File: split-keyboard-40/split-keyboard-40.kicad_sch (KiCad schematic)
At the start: 85 parts, among them SW1 Switch, SW10 Switch, SW11 Switch, SW12 Switch, SW13 Switch, SW14 Switch, SW15 Switch, SW16 Switch, SW17 Switch, SW18 Switch, SW19 Switch, SW2 Switch, SW20 Switch, SW21 Switch, SW22 Switch, SW23 Switch, SW24 Switch, SW25 Switch, SW26 Switch, SW27 Switch, SW28 Switch, SW29 Switch, SW3 Switch, SW30 Switch, SW31 Switch, SW32 Switch, SW33 Switch, SW34 Switch, SW35 Switch, SW36 Switch, SW37 Switch, SW38 Switch, SW39 Switch, SW4 Switch, SW40 Switch, SW41 Switch, SW42 Switch, SW5 Switch, SW6 Switch, SW7 Switch, SW8 Switch, SW9 Switch, U1 Raspberry_Pi_Pico

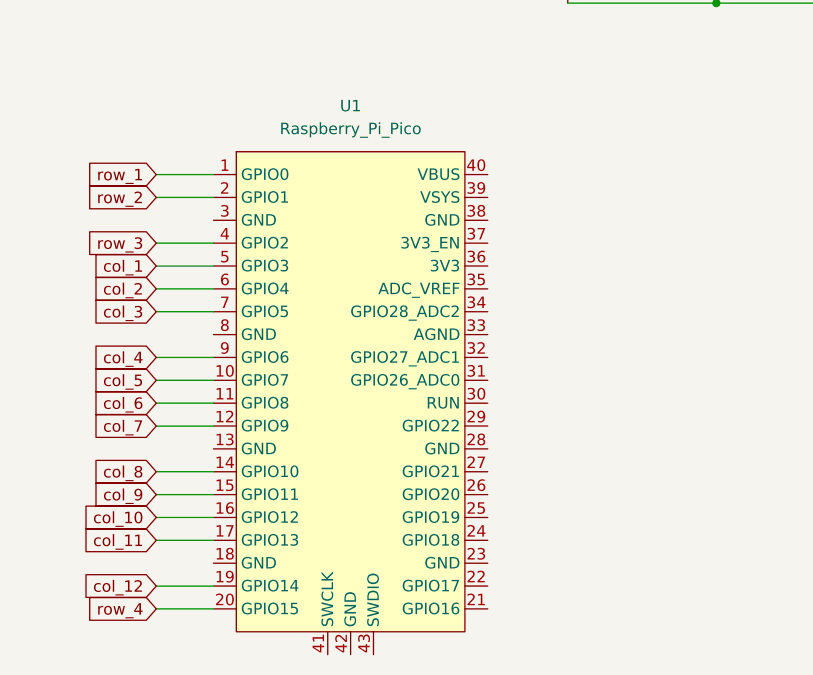
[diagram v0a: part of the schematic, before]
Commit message: few rows
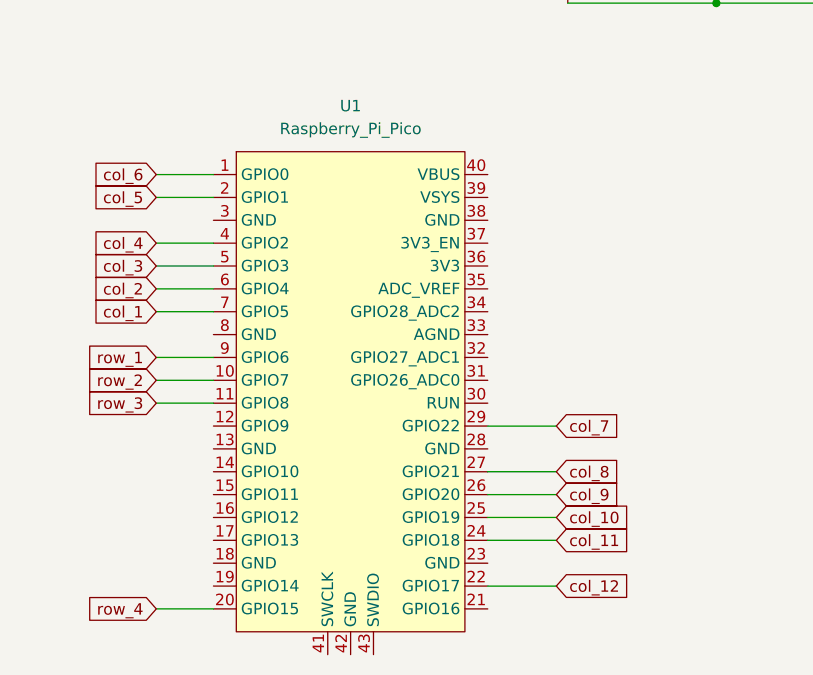
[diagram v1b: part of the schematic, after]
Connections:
- net col_1: now also U1.7 (GPIO5); no longer U1.5 (GPIO3)
- net col_10: now also U1.25 (GPIO19); no longer U1.16 (GPIO12)
- net col_11: now also U1.24 (GPIO18); no longer U1.17 (GPIO13)
- net col_12: now also U1.22 (GPIO17); no longer U1.19 (GPIO14)
- net col_3: now also U1.5 (GPIO3); no longer U1.7 (GPIO5)
- net col_4: now also U1.4 (GPIO2); no longer U1.9 (GPIO6)
- net col_5: now also U1.2 (GPIO1); no longer U1.10 (GPIO7)
- net col_6: now also U1.1 (GPIO0); no longer U1.11 (GPIO8)
- net col_7: now also U1.29 (GPIO22); no longer U1.12 (GPIO9)
- net col_8: now also U1.27 (GPIO21); no longer U1.14 (GPIO10)
- net col_9: now also U1.26 (GPIO20); no longer U1.15 (GPIO11)
- net row_1: now also U1.9 (GPIO6); no longer U1.1 (GPIO0)
- net row_2: now also U1.10 (GPIO7); no longer U1.2 (GPIO1)
- net row_3: now also U1.11 (GPIO8); no longer U1.4 (GPIO2)
